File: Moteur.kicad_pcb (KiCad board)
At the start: 4 copper layers, 30.8 x 16 mm, 54 parts, among them IC1 TPS71501, IC2 TLV710, IC3 MAX3051, IC4 LM5106, IC5 LM5106, IC6 INA282, P1 Bus2, P2 MOTOR, P3 GPIO, P4 CONN_1, P5 DBG, P6 CONN_1, Q1 IRF8721, Q2 IRF8721, Q3 IRF8721, Q4 IRF8721, U1 STM32F303CCT6, X1 16MHz

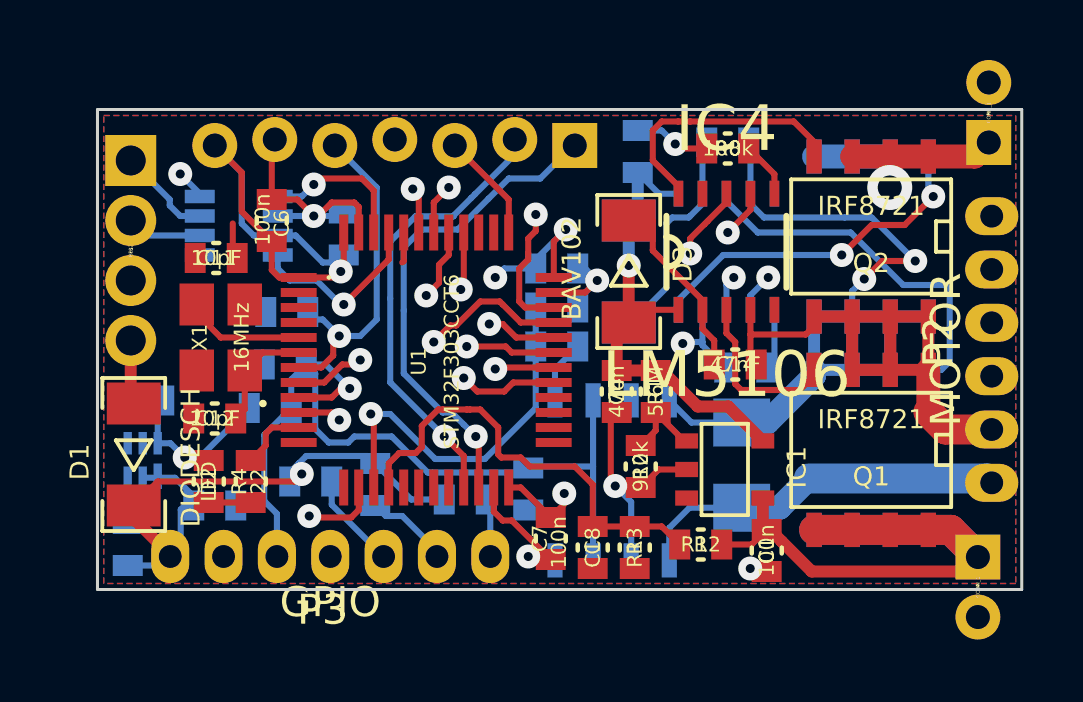
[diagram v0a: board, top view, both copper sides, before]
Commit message: routing, almost done
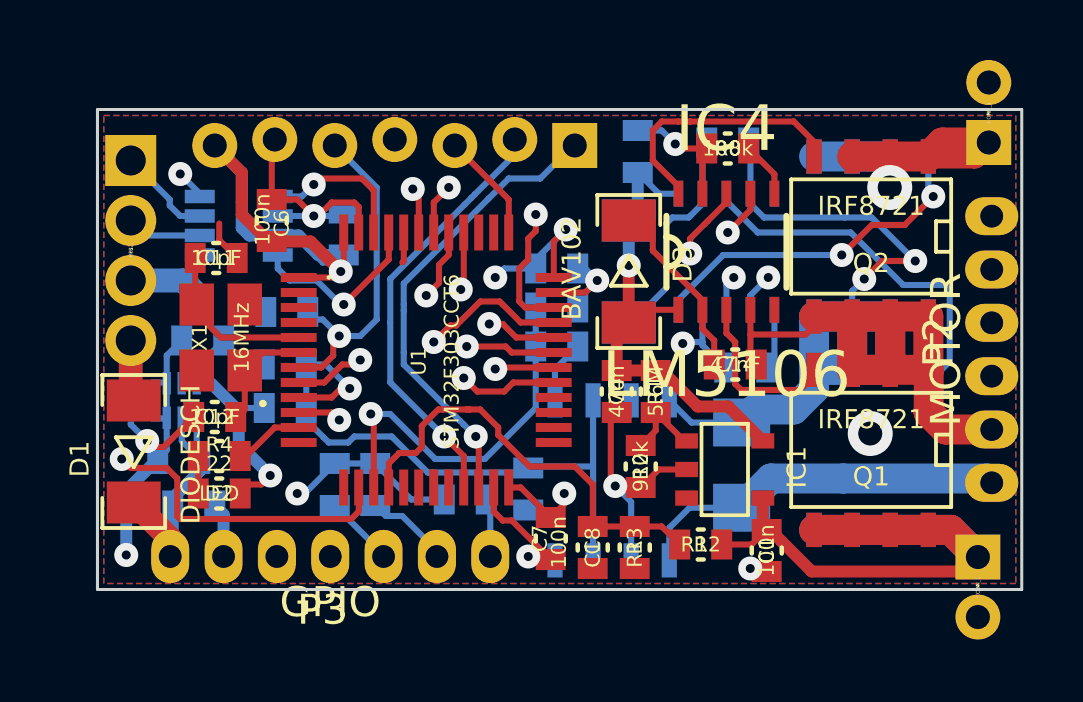
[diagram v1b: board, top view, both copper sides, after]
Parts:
- moved C2 3.32 mm to (125.0, 101.7), turned to 180 degrees
- moved C3 2.83 mm to (125.8, 97.7)
- moved IC2 2.39 mm to (125.1, 99.7)
- moved R4 1.35 mm to (126.3, 101.5), turned to 180 degrees
- moved R3 0.81 mm to (130.2, 102.5), turned to 270 degrees
- moved C17 0.70 mm to (125.5, 103.2)
- moved D2 0.53 mm to (126.3, 102.8), turned to 180 degrees
- moved L1 0.50 mm to (128.6, 100.0)
- moved D1 0.10 mm to (123.5, 101.4)
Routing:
- net GND: track 44.2 -> 74.9 mm, vias 9 -> 12
- net N-0000044: track 29.4 -> 37.8 mm
- net +3.3V: track 49.5 -> 56.9 mm
- net Mot+: track 20.7 -> 26.4 mm
- net CAN_SPEED: track 19.7 -> 22.4 mm
- net N-0000064: track 4.03 -> 5.60 mm
- net +BATT: track 22.3 -> 23.6 mm
- net Rx: track 16.3 -> 15.4 mm
- net GPIO_B: track 14.9 -> 14.1 mm
- net Tx: track 15.1 -> 14.3 mm
- net +5V_protected: track 53.9 -> 54.5 mm
- added copper zone on Inner2.Cu, net GND
